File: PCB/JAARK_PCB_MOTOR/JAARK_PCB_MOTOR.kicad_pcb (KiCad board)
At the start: 2 copper layers, 90 x 90 mm, 55 parts, among them IC1 TPS564242DRLR, IC10 DRV8231DDAR, IC2 PJA3404_R1_00001, IC3 PJA3404_R1_00001, IC4 HIP4080AIBZT, IC5 PJA3404_R1_00001, IC6 PJA3404_R1_00001, IC7 PJA3404_R1_00001, IC8 PJA3404_R1_00001, IC9 DRV8231DDAR, J1 Battery Terminal, Q1 SSM3J334RLF, Q2 SSM3J334RLF, Q3 FMMT619TA, Q4 FMMT619TA, Q5 FMMT619TA, Q6 SSM3J334RLF, Q7 FMMT619TA

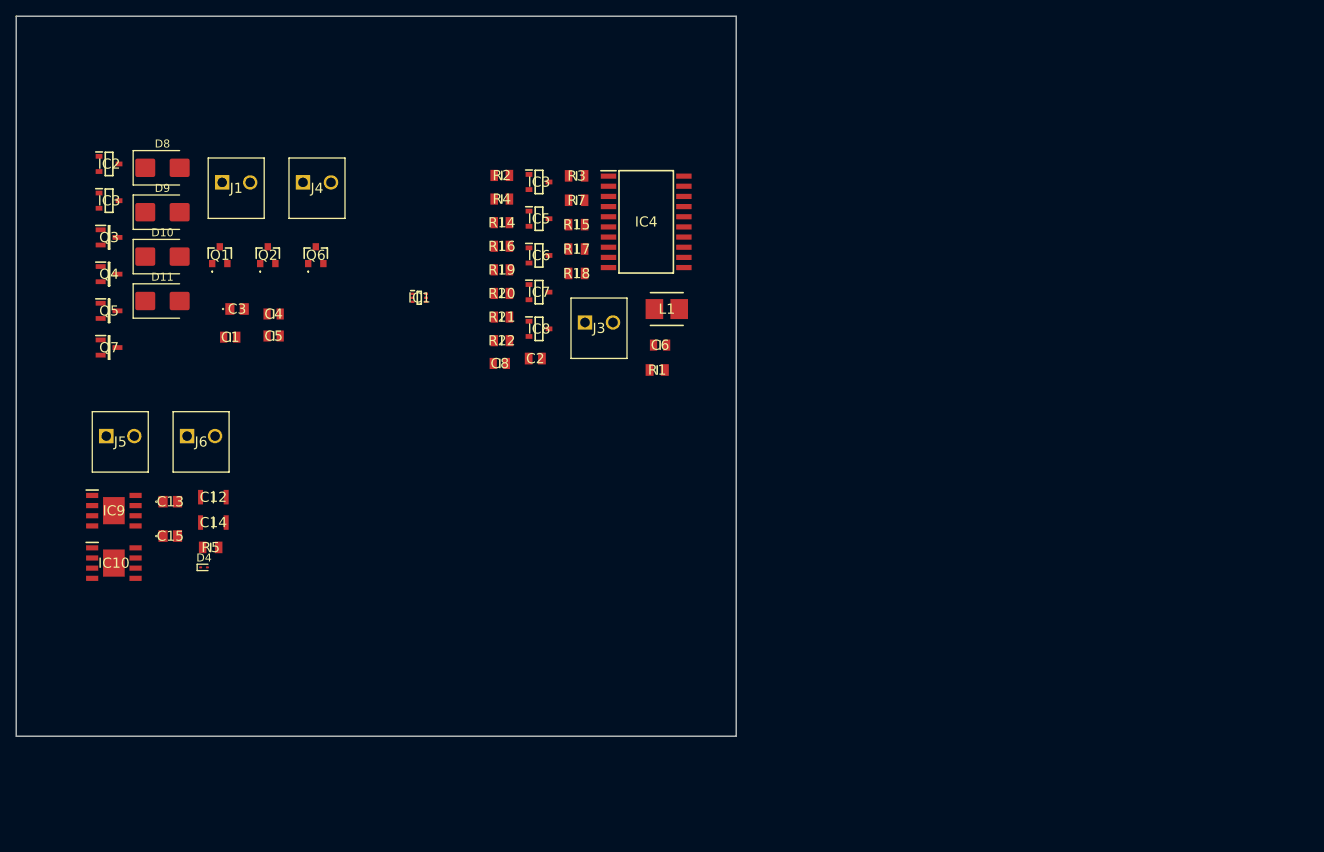
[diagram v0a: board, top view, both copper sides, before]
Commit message: PCB Motor V1 finished.
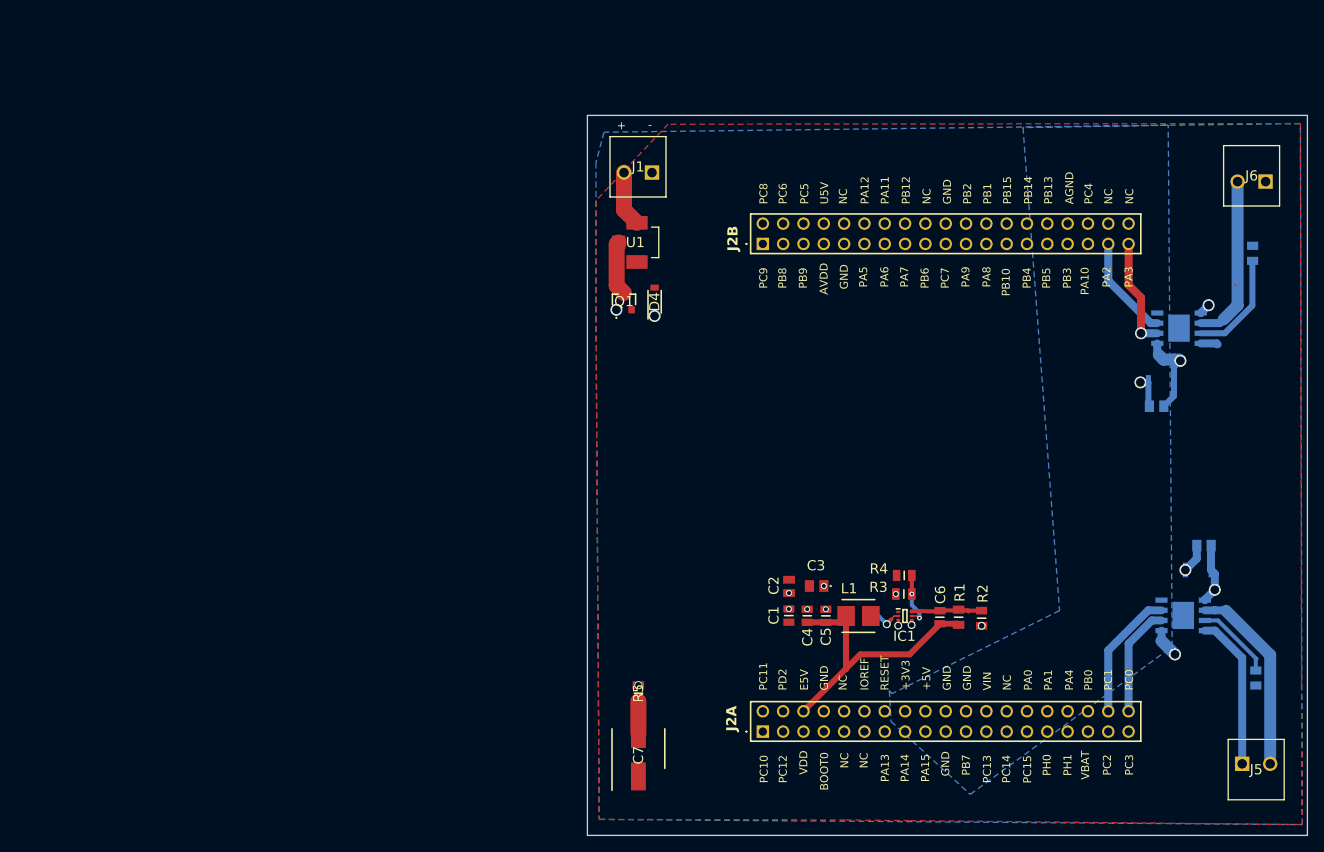
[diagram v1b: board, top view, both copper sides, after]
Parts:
- removed C8: 22uF, JAARK_lib:CAPC2012X95N
- removed D10, D11, D8, D9: S2JTR, Diode_SMD:D_SMB
- removed IC2, IC3, IC5, IC6, IC7, IC8: PJA3404_R1_00001, JAARK_lib:SOT95P240X110-3N
- removed IC3: PJA3404_R1_00001, SSys_Footprints:SOT95P240X110-3N
- removed IC4: HIP4080AIBZT, JAARK_lib:SOIC127P1032X265-20N
- removed J3, J4: ~, JAARK_lib:1984617
- removed Q2, Q6: SSM3J334RLF, JAARK_lib:2SC2712GRLF
- removed Q3, Q4, Q5, Q7: FMMT619TA, JAARK_lib:SOT95P237X112-3N
- removed R14, R16, R21, R22: 260R, JAARK_lib:RESC2012X60N
- removed R15, R17, R18, R7: 5kR, JAARK_lib:RESC2012X50N
- removed R19, R20: 10kR, JAARK_lib:RESC2012X60N
- added C7: 100uF, JAARK_lib:CAPAE660X800N, F.Cu at (106.9, 124.9)
- added J2: Morpho_x2_SSW-119-01-T-D, JAARK_lib:STM_Nucleo_Morpho_x2_Footprint, F.Cu at (122.5, 122.0)
- added R10: 0.2R, JAARK_lib:RESC2013X65N, B.Cu at (184.1, 115.3)
- added R11: 0.2R, JAARK_lib:RESC2013X65N, B.Cu at (183.7, 62.2)
- added U1: 4A, JAARK_lib:3586TR, F.Cu at (106.7, 60.8)
- C12, C13, C14, C15, IC10, IC9: moved to B.Cu
- D4: footprint Diode_SMD:D_SOD-923 -> JAARK_lib:SODFL3616X135N
- moved J5 147.8 mm to (182.4, 126.0)
- moved J6 138.5 mm to (185.3, 53.2), turned to 180 degrees
- moved IC10 136.3 mm to (174.5, 71.5)
- moved IC9 134.3 mm to (175.0, 107.5)
- moved C13 129.3 mm to (177.6, 98.7), turned to 180 degrees
- moved C15 124.4 mm to (171.7, 81.3)
- moved C14 123.2 mm to (176.9, 101.8)
- moved C12 119.3 mm to (172.2, 78.3), turned to 180 degrees
- moved R2 81.6 mm to (149.8, 107.8), turned to 90 degrees
- moved C3 80.3 mm to (129.2, 103.8), turned to 180 degrees
- moved C1 78.0 mm to (125.7, 107.5), turned to 90 degrees
- moved C5 77.4 mm to (130.3, 107.5), turned to -90 degrees
- moved C4 76.6 mm to (128.0, 107.5), turned to -90 degrees
- moved IC1 72.6 mm to (140.2, 107.5)
- moved R4 68.9 mm to (140.1, 102.5)
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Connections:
- IC10 pad 2: /IN1 -> /IN3
- IC10 pad 3: /IN2 -> /IN4
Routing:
- net +5V: track 0.00 -> 36.0 mm
- net Net-(IC9-OUT1): track 0.00 -> 24.1 mm
- net Net-(IC10-OUT1): track 0.00 -> 21.0 mm
- net GND: track 0.00 -> 19.7 mm, vias 0 -> 15
- net Net-(IC9-OUT2): track 0.00 -> 19.3 mm
- net /IN2: track 0.00 -> 16.3 mm
- net /IN3: track 0.00 -> 13.9 mm, vias 0 -> 1
- net /IN1: track 0.00 -> 13.8 mm
- net Net-(IC10-ISEN): track 0.00 -> 13.5 mm
- net +12V: track 0.00 -> 13.0 mm, vias 0 -> 3
- net /IN4: track 0.00 -> 12.9 mm
- net Net-(IC9-ISEN): track 0.00 -> 9.91 mm
- net Net-(IC1-FB): track 0.00 -> 8.70 mm
- net Net-(J1-Pad2): track 0.00 -> 6.94 mm
- net Net-(IC1-EN): track 0.00 -> 6.83 mm, vias 0 -> 2
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- added copper zone on F.Cu, net +12V
- added copper zone on B.Cu, net +3V3
- added copper zone on B.Cu, net GND
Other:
- board text added: "+"
- board text added: "-"
